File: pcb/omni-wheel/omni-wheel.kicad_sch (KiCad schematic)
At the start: 46 parts, among them IC1 AP63301WU-7, IC2 AP63301WU-7, J1 12v TP, J10 Conn_01x01_Pin, J11 Conn_01x01_Pin, J12 5V TP, J13 3.3v TP, J14 GND TP, J15 STLINK, J2 Motor2_output, J3 Motor4_output, J4 Motor3_output, J5 STLINK, J6 Motor1_output, J7 12V Input, J8 Conn_01x01_Pin, J9 Conn_01x01_Pin, SW1 SW_SPST, U1 SN754410NE, U2 SN754410NE, U3 STM32F030R8Tx, U4 CD74HC04E, U6 SN74AC86DR

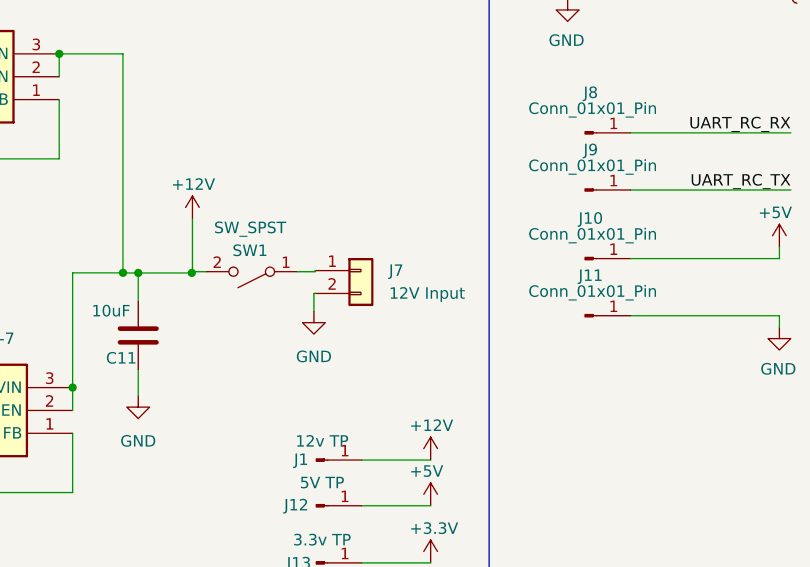
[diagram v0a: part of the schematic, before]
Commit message: purchased this iteration of the board
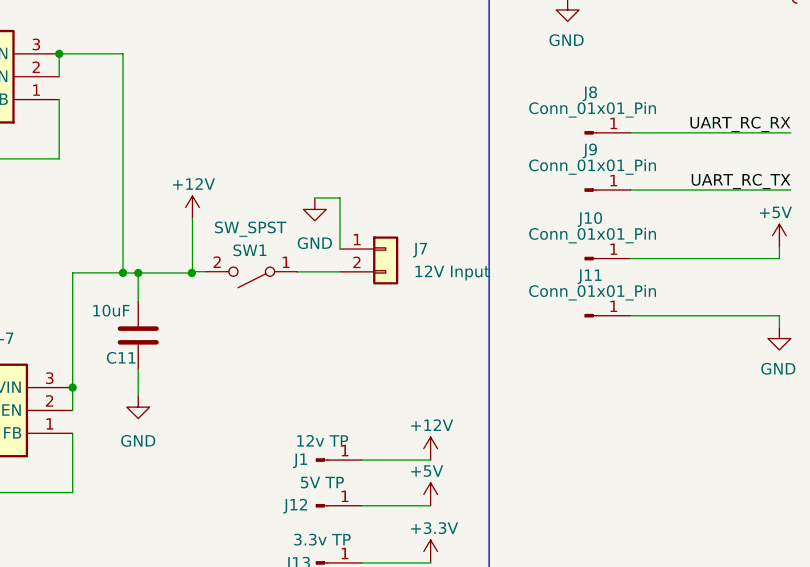
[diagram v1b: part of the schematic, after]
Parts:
- SW1: digikey# (none) -> CWI333-ND; manf# (none) -> GF-123-0054
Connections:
- net GND: now also J7.1 (Pin_1); no longer J7.2 (Pin_2)
- net at SW1.1 (A): now also J7.2 (Pin_2); no longer J7.1 (Pin_1)
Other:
- moved on the sheet: J7
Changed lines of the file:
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@@
 	(wire
 		(pts
-			(xy 121.5026 155.4892) (xy 121.5026 157.4674)
-		)
-		(stroke
-			(width 0)
-			(type default)
-		)
-	)
-	(wire
-		(pts
 			(xy 93.2024 128.87) (xy 100.2871 128.87)
 		)
@@
 	(wire
 		(pts
+			(xy 124.3955 144.8826) (xy 121.6091 144.8826)
+		)
+		(stroke
+			(width 0)
+			(type default)
+		)
+	)
+	(wire
+		(pts
 			(xy 198.3856 63.5124) (xy 202.6638 63.5124)
 		)
@@
 	(wire
 		(pts
+			(xy 119.6717 153.0923) (xy 119.6717 153.0734)
+		)
+		(stroke
+			(width 0)
+			(type default)
+		)
+	)
+	(wire
+		(pts
 			(xy 207.3005 76.2124) (xy 195.8705 76.2124)
 		)
@@
 	(wire
 		(pts
+			(xy 124.3955 150.5523) (xy 124.3955 144.8826)
+		)
+		(stroke
+			(width 0)
+			(type default)
+		)
+	)
+	(wire
+		(pts
 			(xy 134.3015 190.2313) (xy 126.6815 190.2313)
 		)
@@
 	(wire
 		(pts
-			(xy 119.6717 153.0734) (xy 121.6382 153.0734)
-		)
-		(stroke
-			(width 0)
-			(type default)
-		)
-	)
-	(wire
-		(pts
 			(xy 69.2919 161.29) (xy 69.2919 165.9498)
 		)
@@
 	(wire
 		(pts
-			(xy 121.5026 155.4892) (xy 121.6382 155.4892)
-		)
-		(stroke
-			(width 0)
-			(type default)
-		)
-	)
-	(wire
-		(pts
 			(xy 113.03 74.93) (xy 102.87 74.93)
 		)
@@
 	(wire
 		(pts
-			(xy 121.6382 153.0734) (xy 121.6382 152.9492)
-		)
-		(stroke
-			(width 0)
-			(type default)
-		)
-	)
-	(wire
-		(pts
 			(xy 261.62 76.2) (xy 247.65 76.2)
 		)
@@
 	(wire
 		(pts
+			(xy 124.3955 153.0923) (xy 119.6717 153.0923)
+		)
+		(stroke
+			(width 0)
+			(type default)
+		)
+	)
+	(wire
+		(pts
 			(xy 40.1561 140.5536) (xy 40.1561 143.5757)
 		)
@@
 	(symbol
 		(lib_id "Connector_Generic:Conn_01x02")
-		(at 126.7182 152.9492 0)
+		(at 129.4755 150.5523 0)
 		(unit 1)
 		(exclude_from_sim no)
@@
 		(fields_autoplaced yes)
 		(property "Reference" "J7"
-			(at 129.8399 152.9491 0)
+			(at 132.5972 150.5522 0)
 			(effects
 				(font
@@
 		)
 		(property "Value" "12V Input"
-			(at 129.8399 155.4891 0)
+			(at 132.5972 153.0922 0)
 			(effects
 				(font
@@
 		)
 		(property "Footprint" "Connector_AMASS:AMASS_XT30PW-M_1x02_P2.50mm_Horizontal"
-			(at 126.7182 152.9492 0)
+			(at 129.4755 150.5523 0)
 			(effects
 				(font
@@
 		)
 		(property "Datasheet" "~"
-			(at 126.7182 152.9492 0)
+			(at 129.4755 150.5523 0)
 			(effects
 				(font
@@
 		)
 		(property "Description" "Generic connector, single row, 01x02, script generated (kicad-library-utils/schlib/autogen/connector/)"
-			(at 126.7182 152.9492 0)
+			(at 129.4755 150.5523 0)
 			(effects
 				(font
@@
 			)
 		)
+		(property "digikey#" "CWI333-ND"
+			(at 114.5917 153.0734 0)
+			(effects
+				(font
+					(size 1.27 1.27)
+				)
+				(hide yes)
+			)
+		)
+		(property "manf#" "GF-123-0054"
+			(at 114.5917 153.0734 0)
+			(effects
+				(font
+					(size 1.27 1.27)
+				)
+				(hide yes)
+			)
+		)
 		(pin "2"
 		)
@@
 	(symbol
 		(lib_id "power:GND")
-		(at 121.5026 157.4674 0)
+		(at 121.6091 144.8826 0)
 		(unit 1)
 		(exclude_from_sim no)
@@
 		(fields_autoplaced yes)
 		(property "Reference" "#PWR019"
-			(at 121.5026 163.8174 0)
+			(at 121.6091 151.2326 0)
 			(effects
 				(font
@@
 		)
 		(property "Value" "GND"
-			(at 121.5026 162.5327 0)
+			(at 121.6091 149.9479 0)
 			(effects
 				(font
@@
 		)
 		(property "Footprint" ""
-			(at 121.5026 157.4674 0)
+			(at 121.6091 144.8826 0)
 			(effects
 				(font
@@
 		)
 		(property "Datasheet" ""
-			(at 121.5026 157.4674 0)
+			(at 121.6091 144.8826 0)
 			(effects
 				(font
@@
 		)
 		(property "Description" "Power symbol creates a global label with name \"GND\" , ground"
-			(at 121.5026 157.4674 0)
+			(at 121.6091 144.8826 0)
 			(effects
 				(font
